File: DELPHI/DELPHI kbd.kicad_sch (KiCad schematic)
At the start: 86 parts, among them SW1 SW_Push_45deg, SW10 SW_Push_45deg, SW11 SW_Push_45deg, SW12 SW_Push_45deg, SW13 SW_Push_45deg, SW14 SW_Push_45deg, SW15 SW_Push_45deg, SW16 SW_Push_45deg, SW17 SW_Push_45deg, SW18 SW_Push_45deg, SW19 SW_Push_45deg, SW2 SW_Push_45deg, SW20 SW_Push_45deg, SW21 SW_Push_45deg, SW22 SW_Push_45deg, SW23 SW_Push_45deg, SW24 SW_Push_45deg, SW25 SW_Push_45deg, SW26 SW_Push_45deg, SW27 SW_Push_45deg, SW28 SW_Push_45deg, SW29 SW_Push_45deg, SW3 SW_Push_45deg, SW30 SW_Push_45deg, SW31 SW_Push_45deg, SW32 SW_Push_45deg, SW33 SW_Push_45deg, SW34 SW_Push_45deg, SW35 SW_Push_45deg, SW36 SW_Push_45deg, SW37 SW_Push_45deg, SW38 SW_Push_45deg, SW39 SW_Push_45deg, SW4 SW_Push_45deg, SW40 SW_Push_45deg, SW41 SW_Push_45deg, SW42 SW_Push_45deg, SW5 SW_Push_45deg, SW6 SW_Push_45deg, SW7 SW_Push_45deg, SW8 SW_Push_45deg, SW9 SW_Push_45deg, U1 QTPy, U2 QTPy

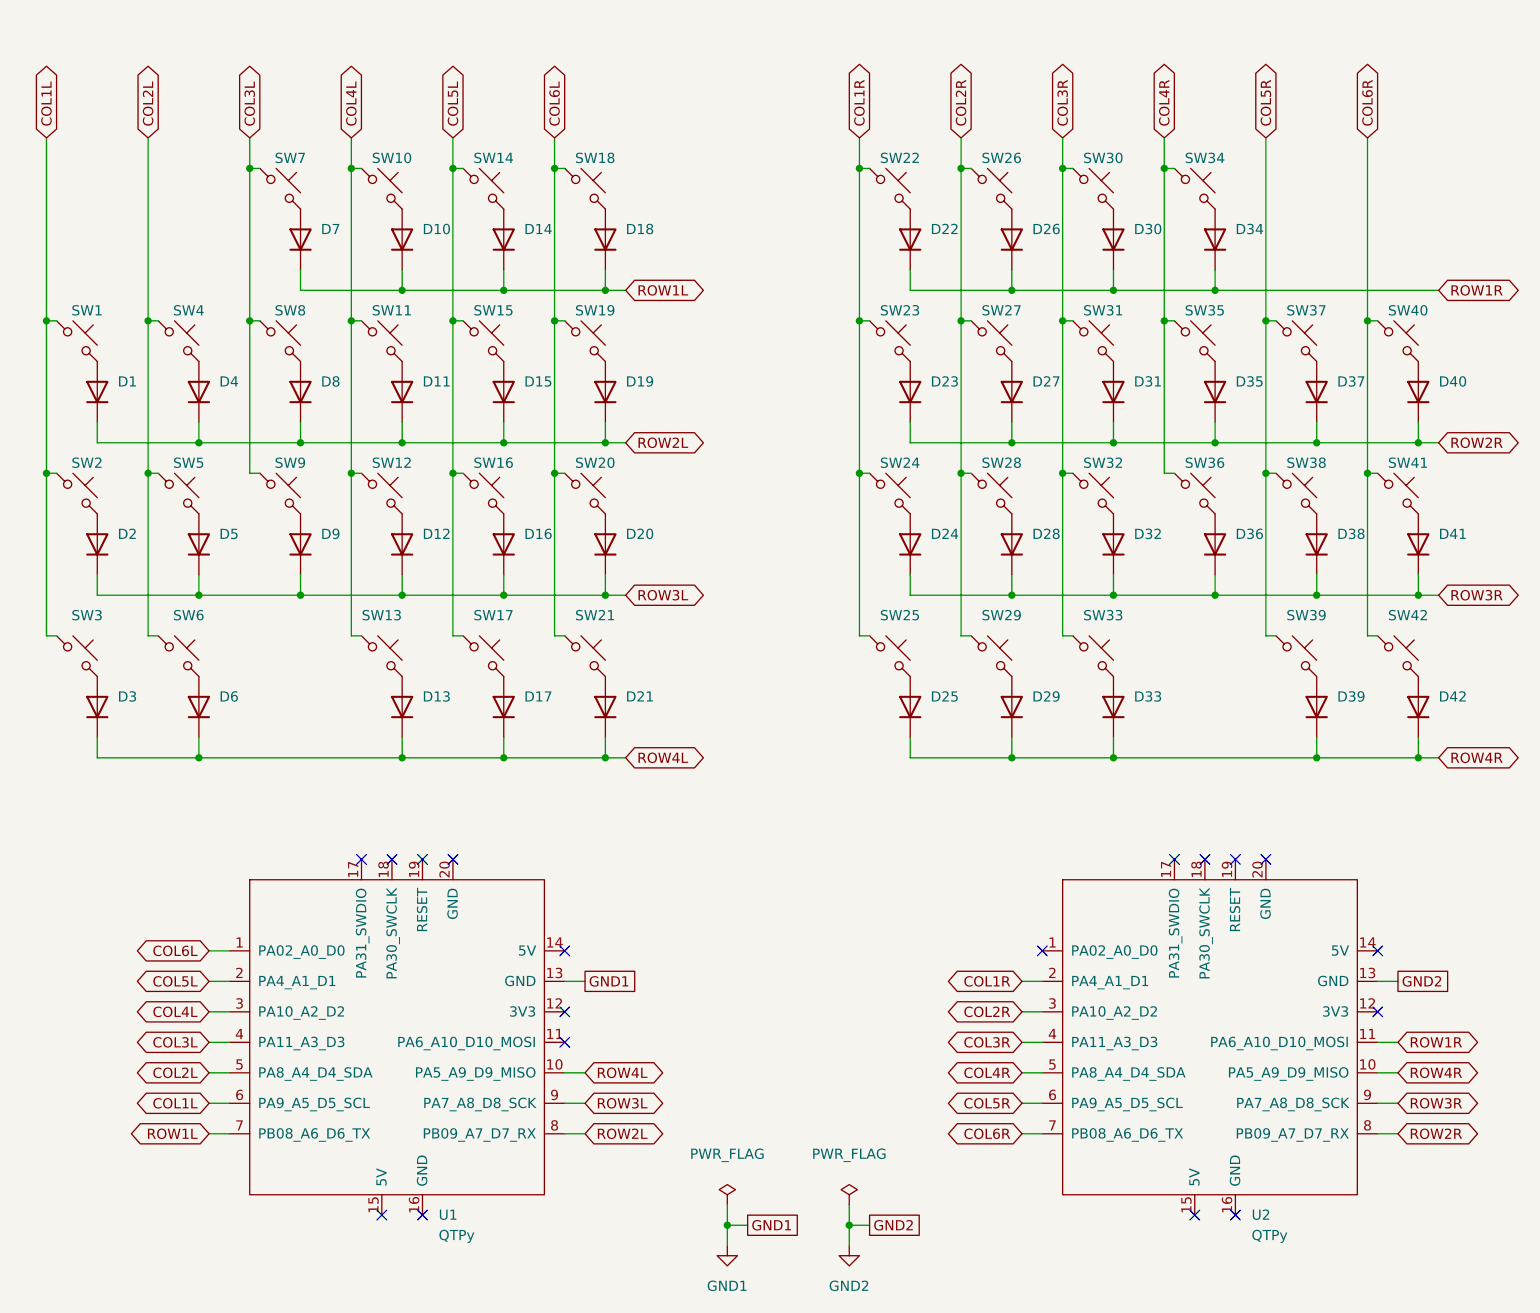
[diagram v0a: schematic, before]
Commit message: Update KiCAD files (specifically the schematic)
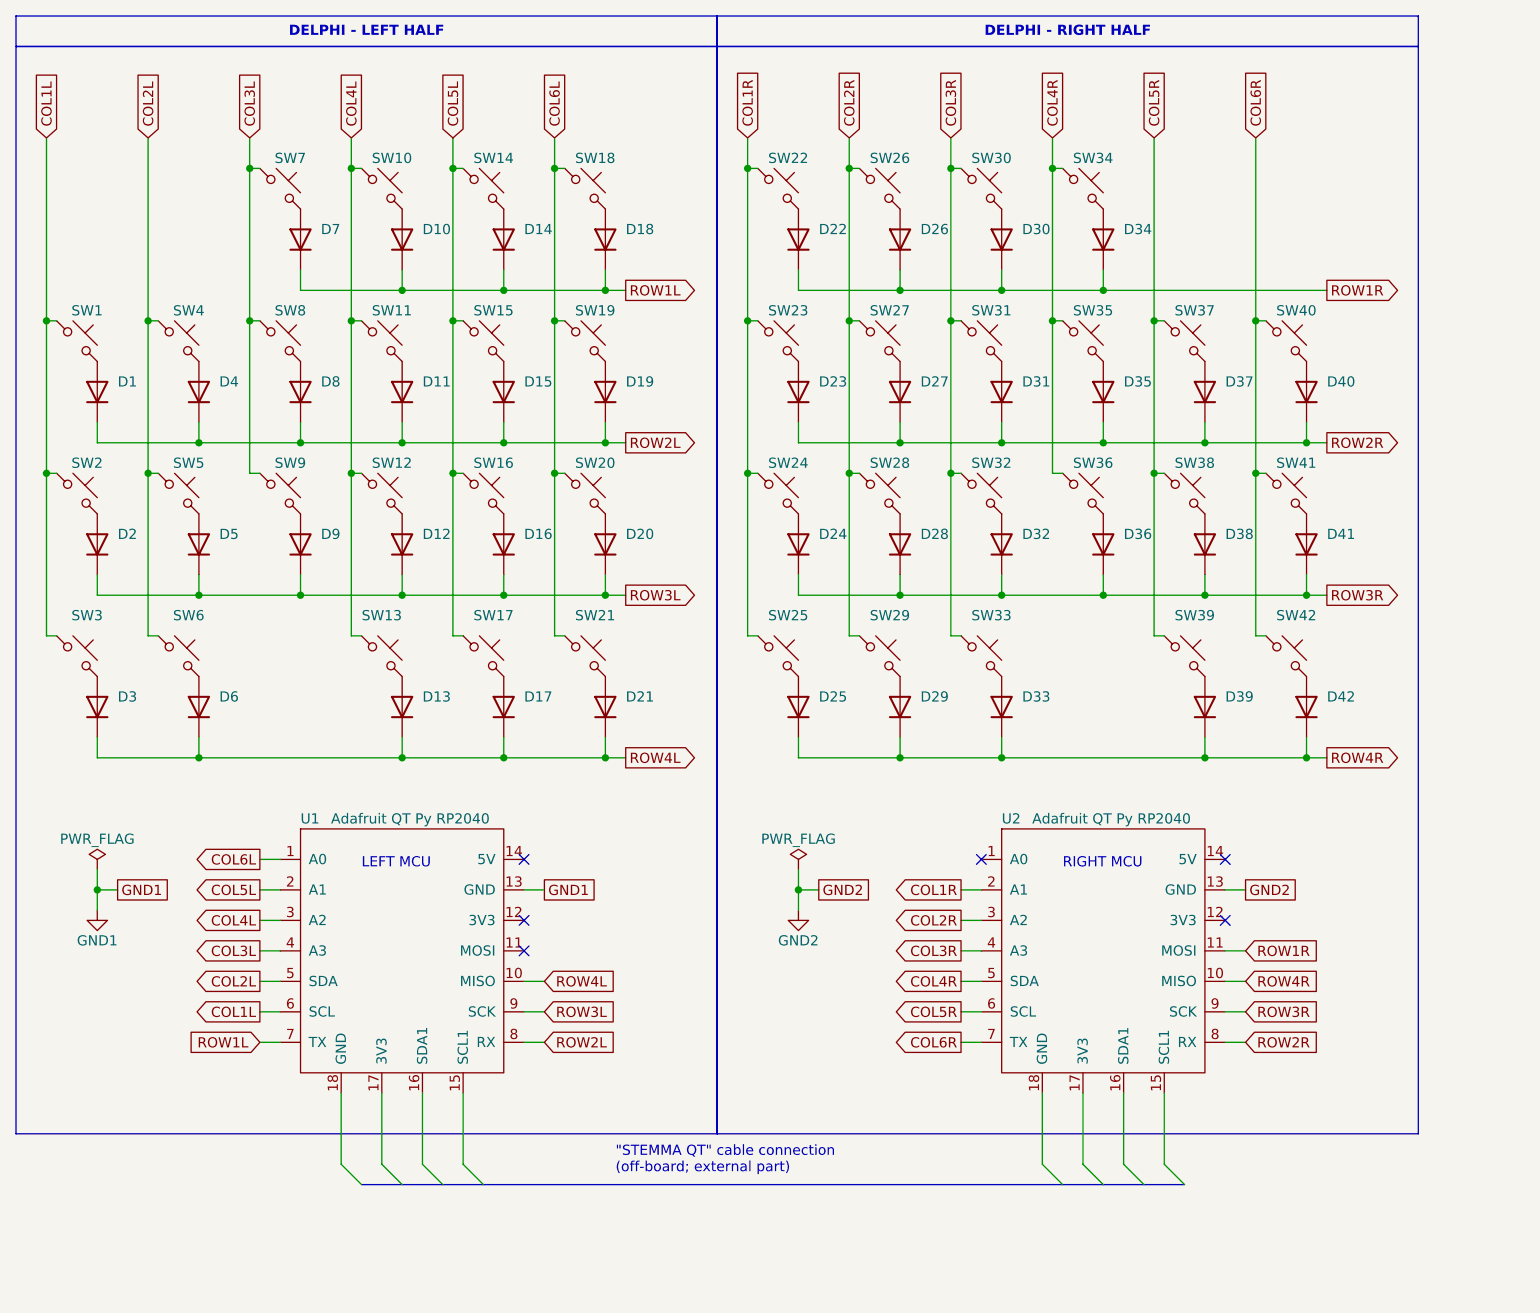
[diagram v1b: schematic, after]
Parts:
- SW1, SW10, SW11, SW12, SW13, SW14, SW15, SW16, SW17, SW18, SW19, SW2, SW20, SW21, SW22, SW23, SW24, SW25, SW26, SW27, SW28, SW29, SW3, SW30, SW31, SW32, SW33, SW34, SW35, SW36, SW37, SW38, SW39, SW4, SW40, SW41, SW42, SW5, SW6, SW7, SW8, SW9: footprint keyswitches:Kailh_socket_PG1350 -> keyswitches.pretty-2:Kailh_socket_PG1350
- U1, U2: value QTPy -> Adafruit QT Py RP2040; footprint Seeeduino XIAO KICAD:Seeeduino XIAO-MOUDLE14P-2.54-21X17.8MM -> Mech Keys:Adafruit QT Py RP2040; symbol Seeeduino XIAO:SeeeduinoXIAO -> Mech Keys:Adafruit_QT_Py_RP2040
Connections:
- no-connect marks 18 -> 6
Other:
- note added: ""STEMMA QT" cable connection (off-board; external part)"
- note added: "LEFT MCU"
- note added: "RIGHT MCU"
- moved on the sheet: D22, D23, D24, D25, D26, D27, D28, D29, D30, D31, D32, D33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
